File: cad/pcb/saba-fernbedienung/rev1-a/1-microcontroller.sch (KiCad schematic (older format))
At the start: 12 parts, among them J201 Conn_ARM_JTAG_SWD_10, Q201 BC856, U201 DOIT-DEVKITV1-ESP32-WROOM-32

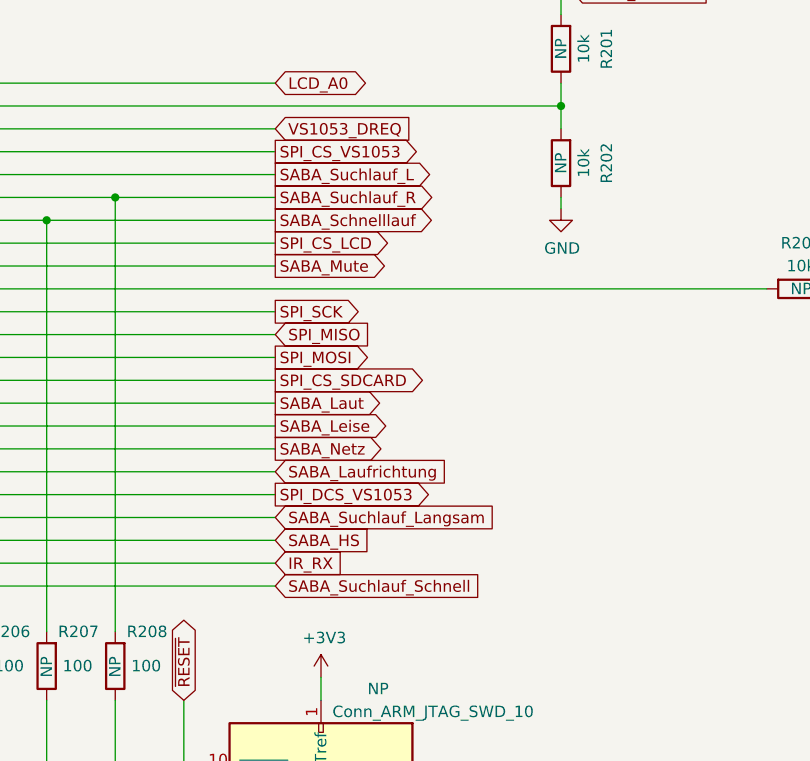
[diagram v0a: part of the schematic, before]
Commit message: Sicherung
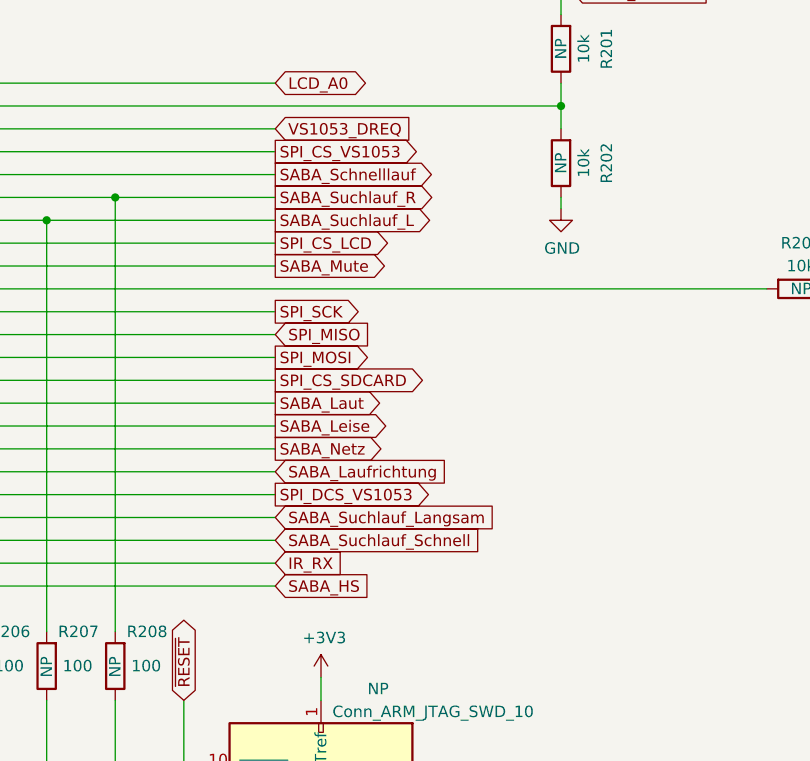
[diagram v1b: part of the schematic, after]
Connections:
- net SABA_HS: now also U201.17 (SENSOR_VP/IO36); no longer U201.19 (IO34)
- net SABA_Schnelllauf: now also R205.2, U201.27 (IO12); no longer R207.2, U201.26 (IO14)
- net SABA_Suchlauf_L: now also R207.2, U201.26 (IO14); no longer R205.2, U201.27 (IO12)
- net SABA_Suchlauf_Schnell: now also U201.19 (IO34); no longer U201.17 (SENSOR_VP/IO36)
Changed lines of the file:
@@
 Wire Wire Line
 	8400 2500 8400 2600
-Text GLabel 5550 3900 2    50   Input ~ 0
+Text GLabel 5550 4100 2    50   Input ~ 0
 SABA_HS
 Wire Wire Line
@@
 Text GLabel 5550 2400 2    50   Output ~ 0
 SABA_Suchlauf_R
-Text GLabel 5550 2300 2    50   Output ~ 0
+Text GLabel 5550 2500 2    50   Output ~ 0
 SABA_Suchlauf_L
 Wire Wire Line
@@
 Text GLabel 5550 3800 2    50   Input ~ 0
 SABA_Suchlauf_Langsam
-Text GLabel 5550 4100 2    50   Input ~ 0
+Text GLabel 5550 3900 2    50   Input ~ 0
 SABA_Suchlauf_Schnell
 $Comp
@@
 	1    0    0    -1
 $EndComp
-Text GLabel 5550 2500 2    50   Output ~ 0
+Text GLabel 5550 2300 2    50   Output ~ 0
 SABA_Schnelllauf
 Wire Wire Line

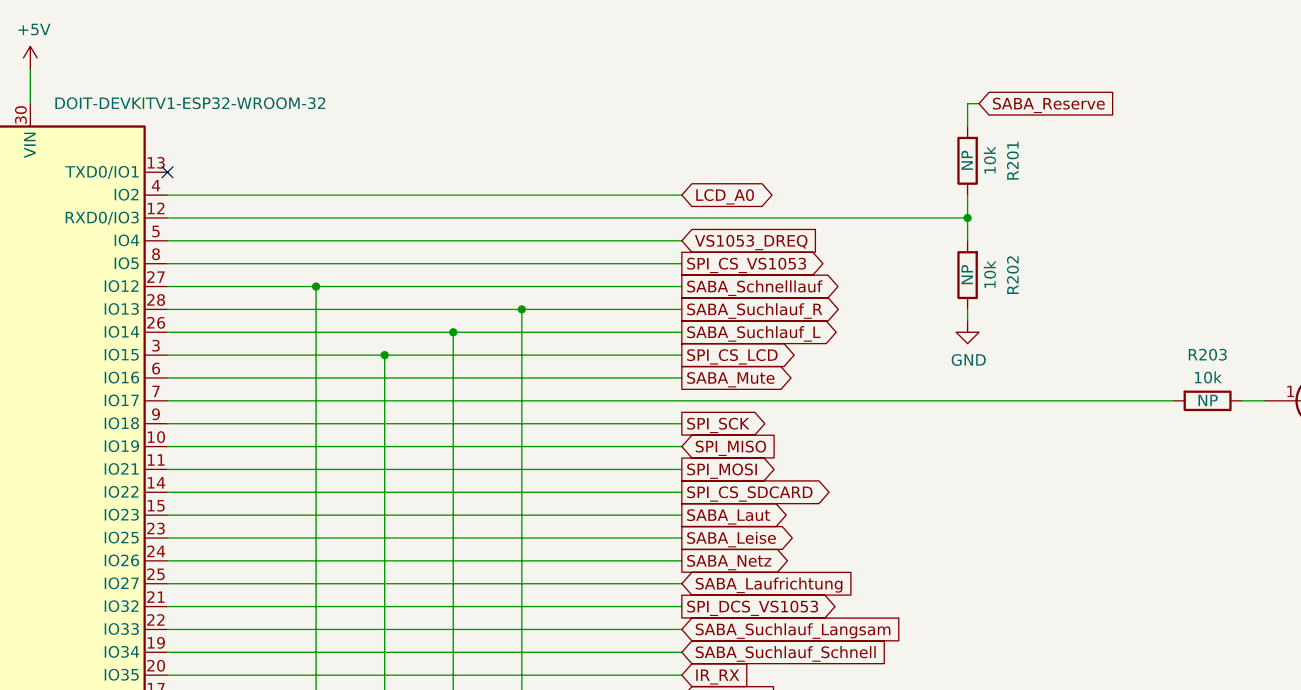
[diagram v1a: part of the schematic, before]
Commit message: Sicherung
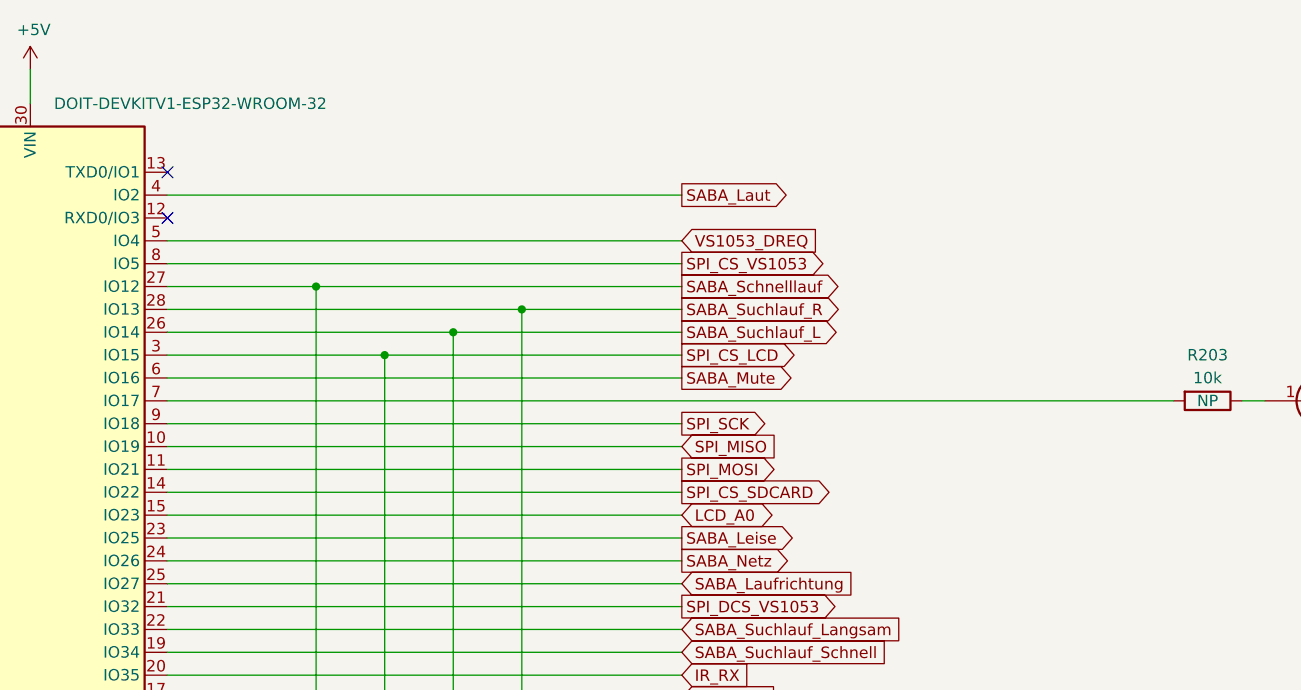
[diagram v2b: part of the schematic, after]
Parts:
- removed R201, R202: 10k, Resistor_SMD:R_0603_1608Metric, symbol Device:R
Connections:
- net LCD_A0: now also U201.15 (IO23); no longer U201.4 (IO2)
- net SABA_Laut: now also U201.4 (IO2); no longer U201.15 (IO23)
- no-connect marks 1 -> 2
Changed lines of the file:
@@
 Wire Wire Line
 	5550 3700 3300 3700
-Text GLabel 5550 1900 2    50   BiDi ~ 0
+Text GLabel 5550 3300 2    50   BiDi ~ 0
 LCD_A0
 Text GLabel 5550 2600 2    50   Output ~ 0
@@
 Text GLabel 5550 2700 2    50   Output ~ 0
 SABA_Mute
-Wire Wire Line
-	5550 2700 3300 2700
-Text GLabel 5550 3300 2    50   Output ~ 0
+Text GLabel 5550 1900 2    50   Output ~ 0
 SABA_Laut
 Text GLabel 5550 3400 2    50   Output ~ 0
@@
 	1    0    0    1
 $EndComp
-$Comp
-L Device:R R201
-U 1 1 60A2E32A
-P 6800 1750
-F 0 "R201" V 6600 1750 50  0000 C CNN
-F 1 "10k" V 6700 1750 50  0000 C CNN
-F 2 "Resistor_SMD:R_0603_1608Metric" V 6730 1750 50  0001 C CNN
-F 3 "~" H 6800 1750 50  0001 C CNN
-F 4 "NP" V 6800 1750 50  0000 C CNN "Placement"
-	1    6800 1750
-	-1   0    0    1
-$EndComp
-$Comp
-L Device:R R202
-U 1 1 60A2EA0B
-P 6800 2250
-F 0 "R202" V 6600 2250 50  0000 C CNN
-F 1 "10k" V 6700 2250 50  0000 C CNN
-F 2 "Resistor_SMD:R_0603_1608Metric" V 6730 2250 50  0001 C CNN
-F 3 "~" H 6800 2250 50  0001 C CNN
-F 4 "NP" V 6800 2250 50  0000 C CNN "Placement"
-	1    6800 2250
-	-1   0    0    1
-$EndComp
-Wire Wire Line
-	3300 2000 6800 2000
-Wire Wire Line
-	6800 1900 6800 2000
-Connection ~ 6800 2000
-Wire Wire Line
-	6800 2000 6800 2100
-Wire Wire Line
-	6800 2400 6800 2450
-Text GLabel 6850 1500 2    50   Input ~ 0
-SABA_Reserve
-Wire Wire Line
-	6800 1600 6800 1500
-$Comp
-L power:GND #PWR0202
-U 1 1 60A7B96C
-P 6800 2450
-F 0 "#PWR0202" H 6800 2200 50  0001 C CNN
-F 1 "GND" H 6805 2277 50  0000 C CNN
-F 2 "" H 6800 2450 50  0001 C CNN
-F 3 "" H 6800 2450 50  0001 C CNN
-	1    6800 2450
-	1    0    0    -1
-$EndComp
-Wire Wire Line
-	6800 1500 6850 1500
+Wire Wire Line
+	5550 2700 3300 2700
+NoConn ~ 3300 2000
 $EndSCHEMATC
